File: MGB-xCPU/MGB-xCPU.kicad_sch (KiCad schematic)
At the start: 61 parts, among them P1 GameBoy_Cartridge, U1 CPU MGB, U2 LH52A64N, U6 PST9135N, X1 4.194304 MHz

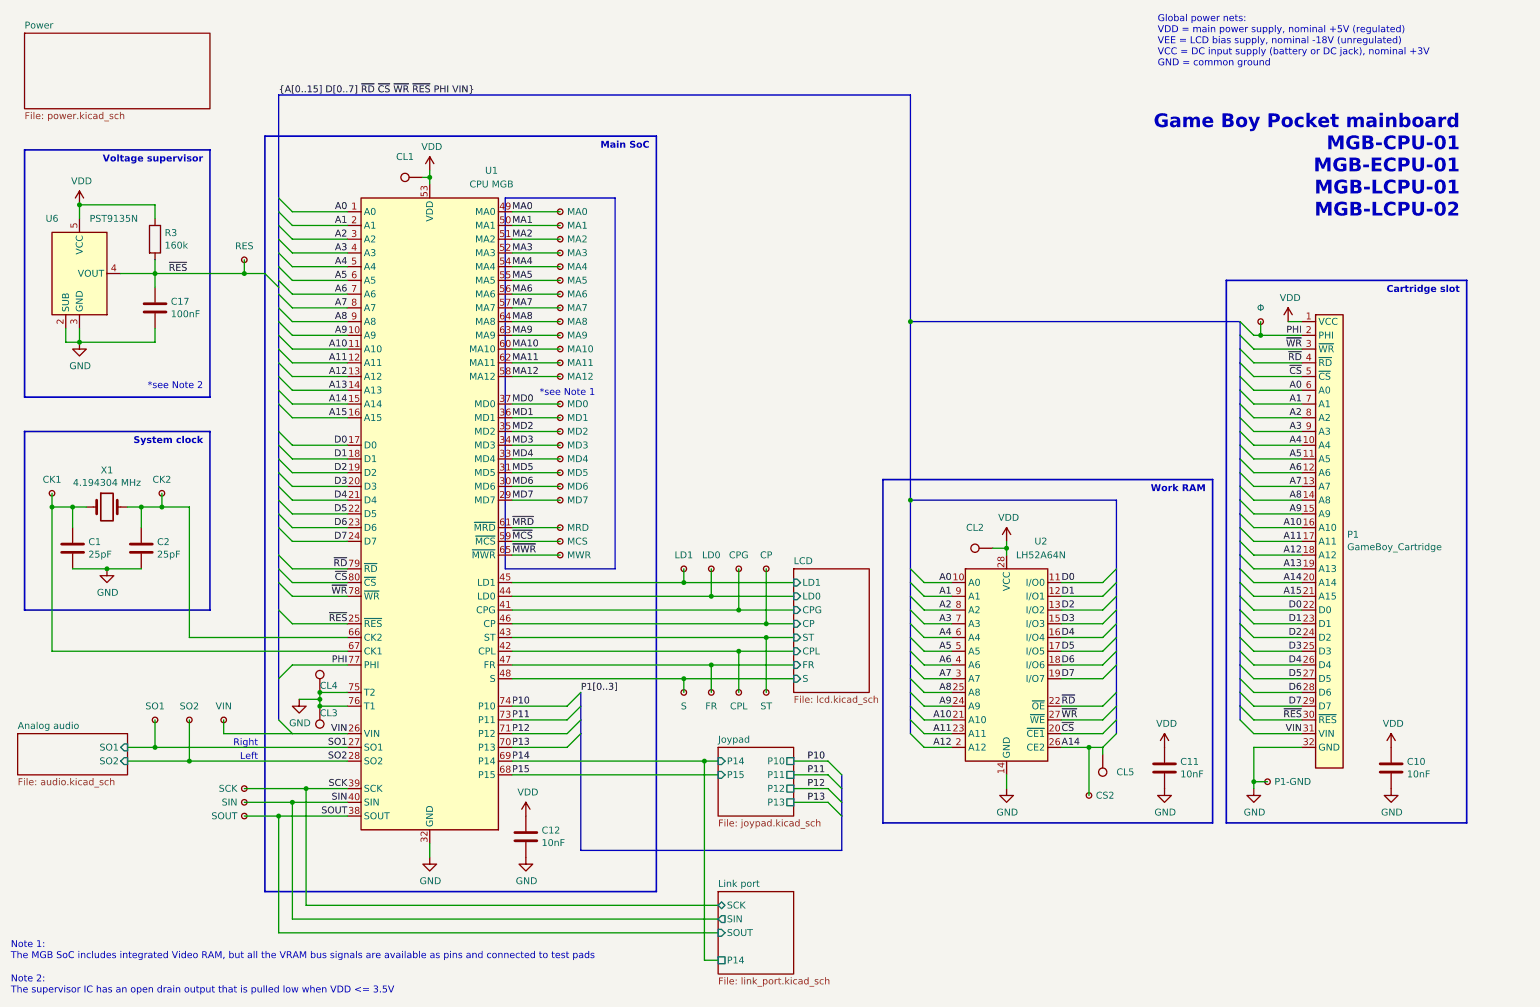
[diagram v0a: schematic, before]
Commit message: Update to latest KiCad
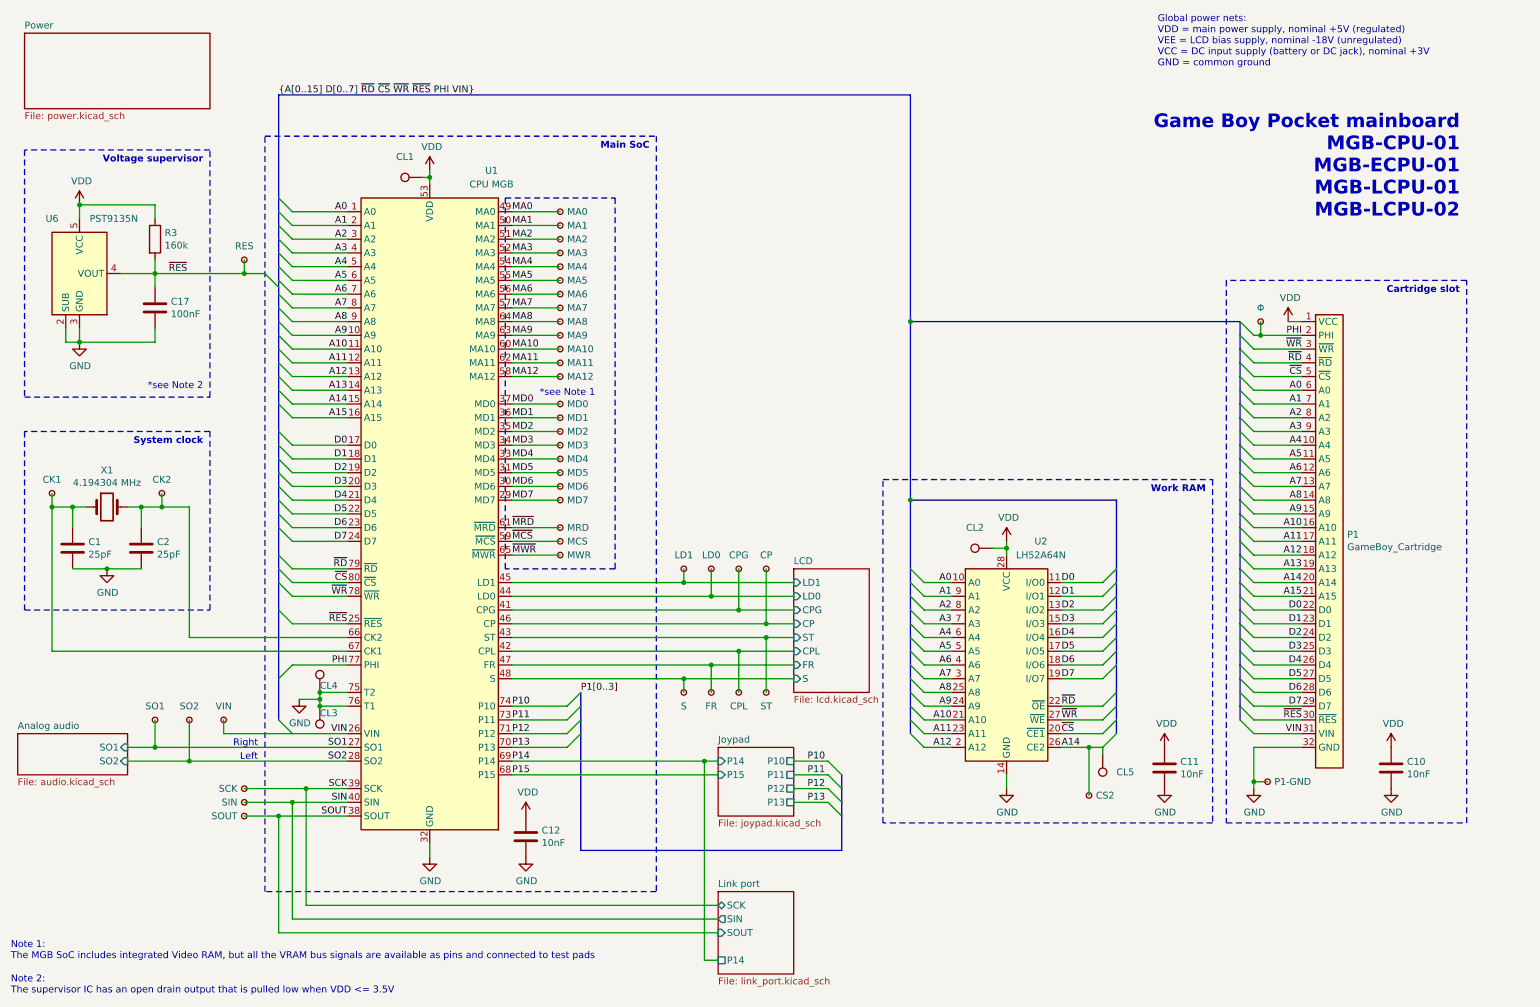
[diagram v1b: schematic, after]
